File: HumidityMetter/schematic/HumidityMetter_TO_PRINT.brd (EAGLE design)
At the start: 100 x 68 mm, 66 parts, among them IC1 LM317, IC2 LM317, IC3 STM32F103C8T6, IC4 AM2320, J1 0, J2 0, J3 0, J4 0, K1 POWER_ON, T1 BSS84, T2 BC847, X1 +9V, X2 GND, X3 ISP

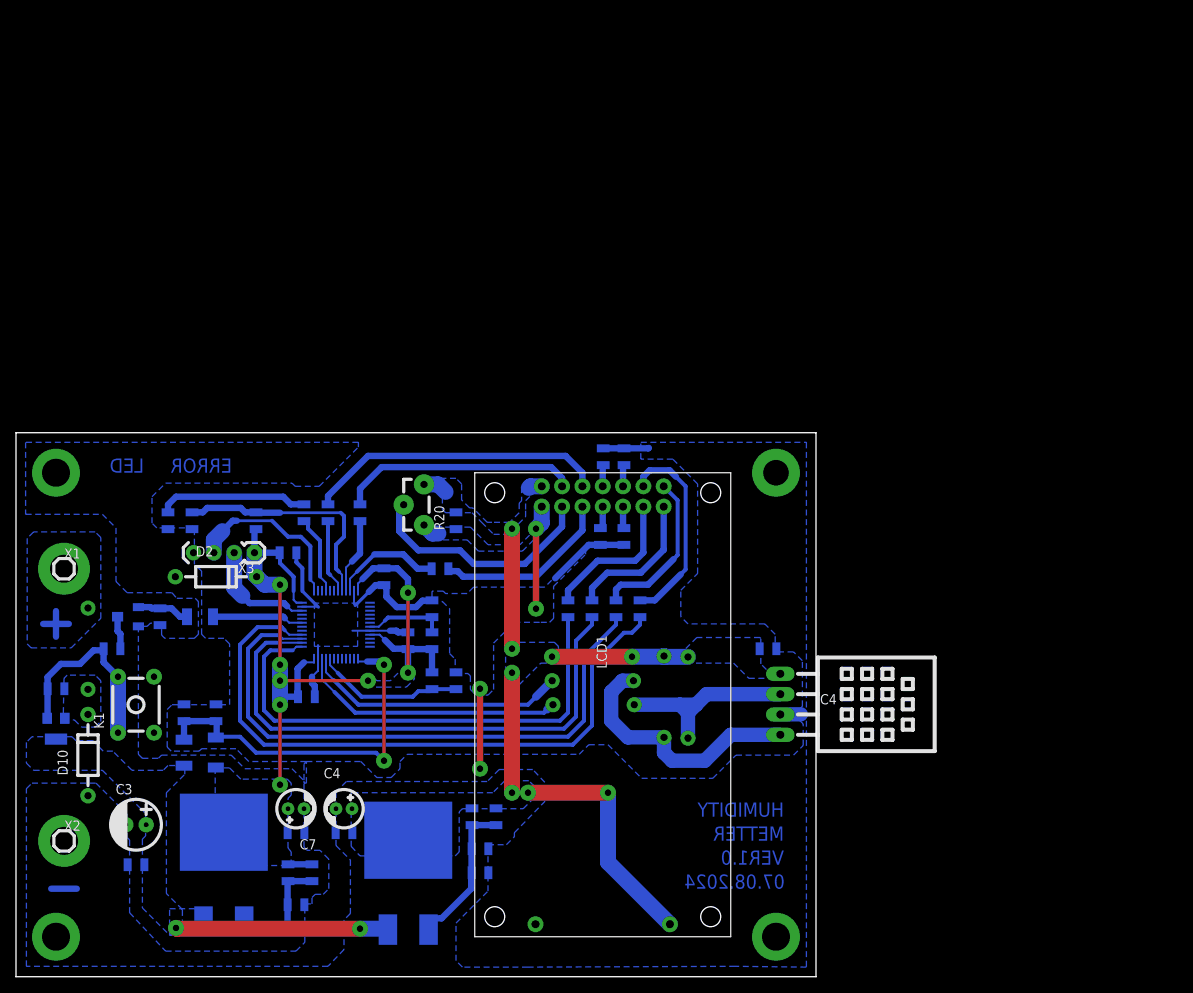
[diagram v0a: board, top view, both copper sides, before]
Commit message: Himidity metter. Board routed. Fix tiny problems.
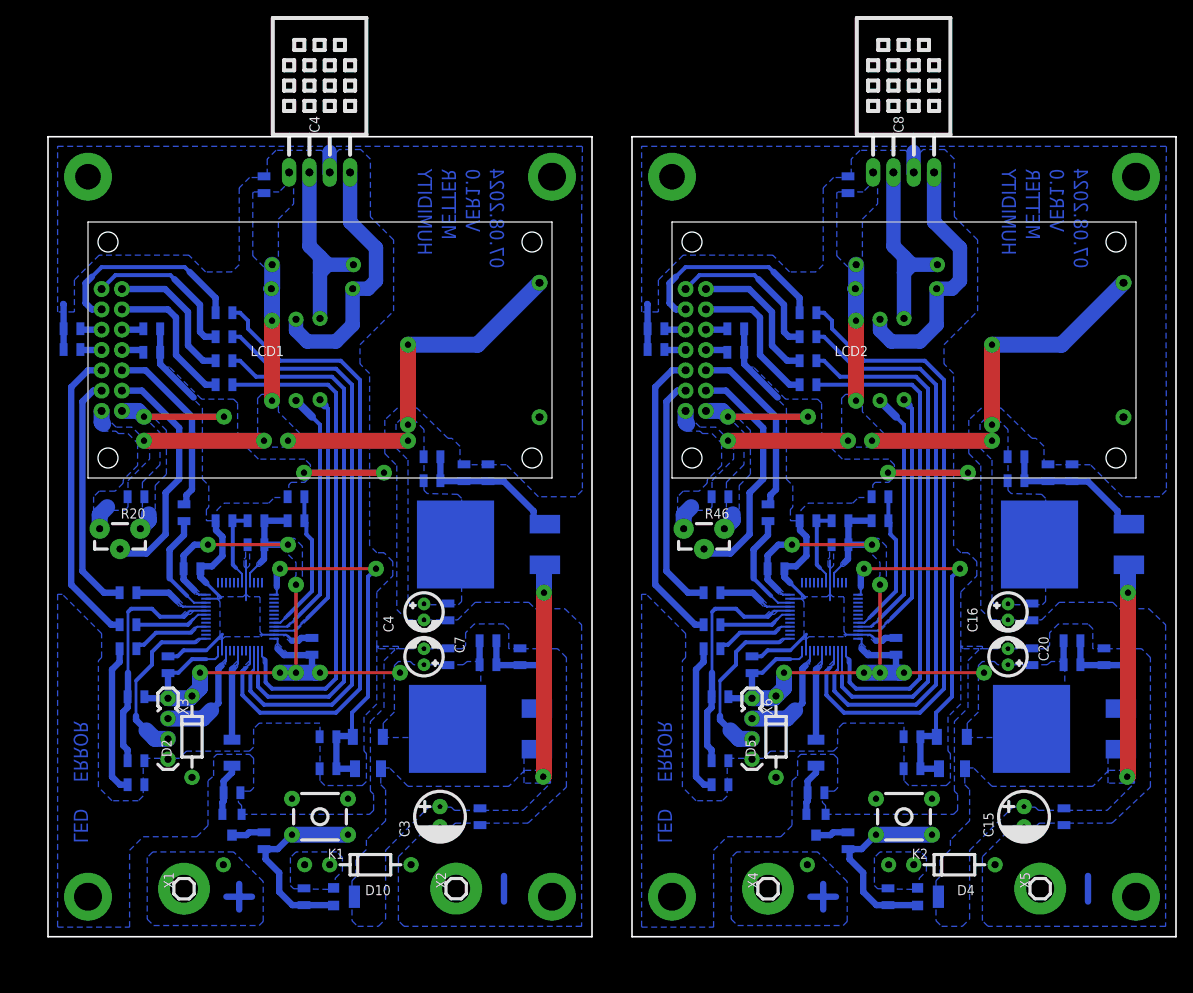
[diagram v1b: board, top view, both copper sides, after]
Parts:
- added C15: 100uFx16V, __MyCommonLib1:CE_6.3MM
- added C16, C20: 10uF x 10V, __MyCommonLib1:CE_5.2MM
- added C17, C18, C19, C21, C22, C23, C24, C25, C26, C27, C28: 0.1uF, __MyCommonLib1:RSMD_0805
- added D3: LL4148, __MyCommonLib1:SOD-80
- added D4, D5: 1N4007, __MyCommonLib1:DO-41_10MM
- added IC5: STM32F103C8T6, __MyCommonLib1:LQFP48
- added IC6, IC7: LM317, __MyCommonLib1:D2PAK
- added IC8: AM2320, __MyCommonLib1:AM2320_HOR
- added J5, J6, J7, J8: 0, __MyCommonLib1:RSMD_0805
- added K2: POWER_ON, __MyCommonLib1:KEY_7X4.5
- added LCD2: LCD_0802B, __MyCommonLib1:LCD_0802B(CHINA_CLONE)
- added LED2: ERROR(RED), __MyCommonLib1:LED_0805
- added R34: 1 Ohm, __MyCommonLib1:R0207
- added R35, R37, R59: 10K, __MyCommonLib1:RSMD_0805
- added R36, R38, R66: 1K0, __MyCommonLib1:RSMD_0805
- added R39: 3K0, __MyCommonLib1:RSMD_0805
- added R40, R43, R64, R65: *, __MyCommonLib1:RSMD_0805
- added R41: 3K9, __MyCommonLib1:RSMD_0805
- added R42: 2K2, __MyCommonLib1:RSMD_0805
- added R44: 1K0, __MyCommonLib1:RSMD_1206_BIG_GAP
- added R45, R47, R48, R49, R54, R55, R56: 390R, __MyCommonLib1:RSMD_0805
- added R46: 10K, __MyCommonLib1:R_ADJ_STAND
- added R50, R51, R52, R53: 2K0, __MyCommonLib1:RSMD_0805
- added R57: 18K, __MyCommonLib1:RSMD_1206_BIG_GAP
- added R58: 6K8, __MyCommonLib1:RSMD_0805
- added R60, R61: 4K7, __MyCommonLib1:R0207
- added R62, R63: 200R, __MyCommonLib1:R0207
- added T3: BSS84, __MyCommonLib1:SOT23
- added T4: BC847, __MyCommonLib1:SOT23_SMALL_PADS
- added X4: +9V, __MyCommonLib1:PIN1X1_D3.5MM
- added X5: GND, __MyCommonLib1:PIN1X1_D3.5MM
- added X6: ISP, __MyCommonLib1:PIN4X1_2.54MM
- moved IC4 94.3 mm to (34.0, 100.0), turned to 90 degrees
- moved C1 85.6 mm to (27.0, 94.0), turned to 270 degrees
- moved R26 71.6 mm to (33.1, 84.0), turned to 180 degrees
- moved R16 70.8 mm to (3.00, 76.0), turned to 0 degrees
- moved R18 67.7 mm to (3.00, 73.4), turned to 0 degrees
- moved R27 67.4 mm to (33.0, 81.0), turned to 180 degrees
- moved R17 64.5 mm to (13.0, 76.0), turned to 180 degrees
- moved R14 63.8 mm to (22.0, 78.0), turned to 180 degrees
- moved R19 60.6 mm to (13.0, 73.0), turned to 180 degrees
- moved R12 59.6 mm to (22.0, 75.0), turned to 180 degrees
- moved R13 55.5 mm to (22.0, 72.0), turned to 180 degrees
- moved R28 55.1 mm to (34.0, 72.2), turned to 90 degrees
- moved R29 54.6 mm to (31.0, 72.1), turned to 90 degrees
- moved R15 51.3 mm to (22.0, 69.0), turned to 180 degrees
- moved R6 50.0 mm to (55.0, 58.0), turned to 90 degrees
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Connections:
- new net +3.3V1: C19.PAD_1, C20.PLUS, C23.PAD_1, C24.PAD_1, C25.PAD_1, C26.PAD_1, D3.CATHODE, D5.CATHODE, IC5.24, IC5.36, IC5.48, IC5.9, IC7.2, J5.PAD_0, J7.PAD_0, R42.PAD_1, R59.PAD_0, R64.PAD_1, X6.1
- new net +5V1: C16.PLUS, C18.PAD_1, C21.PAD_1, C28.PAD_1, IC6.2, IC8.1, LCD2.2, LCD2.A, R38.PAD_1, R46.3, R60.PAD_0, R61.PAD_0, R65.PAD_1
- new net ADC_9V1: C22.PAD_1, D3.ANODE, IC5.13, R57.PAD_1, R58.PAD_0
- new net BOOT2: IC5.20, J7.PAD_1, J8.PAD_0
- new net BOOT3: IC5.44, J5.PAD_1, J6.PAD_0
- new net ERROR_LED1: IC5.40, R66.PAD_0
- new net GND1: C15.MINUS, C16.MINUS, C17.PAD_0, C18.PAD_0, C19.PAD_0, C20.MINUS, C21.PAD_0, C22.PAD_0, C23.PAD_0, C24.PAD_0, C25.PAD_0, C26.PAD_0, C27.PAD_0, C28.PAD_0, D4.ANODE, D5.ANODE, IC5.23, IC5.35, IC5.47, IC5.8, IC8.3, J6.PAD_1, J8.PAD_1, K2.1, K2.2, LCD2.1, LCD2.K, LED2.CATHODE, R37.PAD_1, R39.PAD_1, R40.PAD_1, R41.PAD_1, R43.PAD_1, R46.1, R50.PAD_1, R51.PAD_1, R52.PAD_1, R53.PAD_1, R58.PAD_1, T4.2, X5.1, X6.4
- new net I2C_SCL1: IC5.21, R63.PAD_0
- new net I2C_SDA1: IC5.22, R62.PAD_0
- new net LCD_D1: IC5.27, R45.PAD_1
- new net LCD_D2: IC5.26, R47.PAD_1
- new net LCD_D3: IC5.28, R48.PAD_1
- new net LCD_D8: IC5.25, R49.PAD_1
- new net LCD_E1: IC5.43, R54.PAD_1
- new net LCD_R/~W1: IC5.46, R55.PAD_1
- new net LCD_RS1: IC5.45, R56.PAD_1
- new net N$24: R34.PAD1, X4.1
- new net N$25: D4.CATHODE, R34.PAD_0, R35.PAD_0, T3.2
- new net N$26: K2.3, K2.4, R35.PAD_1, R36.PAD_0, T3.1
- new net N$27: R36.PAD_1, T4.3
- new net N$29: R37.PAD_0, R44.PAD_1, T4.1
- new net N$31: C15.PLUS, C17.PAD_1, IC6.3, IC7.3, R57.PAD_0, T3.3
- new net N$32: IC6.1, R38.PAD_0, R39.PAD_0, R40.PAD_0, R65.PAD_0
- new net N$33: IC7.1, R41.PAD_0, R42.PAD_0, R43.PAD_0, R64.PAD_0
- new net N$34: LCD2.14, R45.PAD_0
- new net N$35: LCD2.13, R47.PAD_0
- new net N$36: LCD2.12, R48.PAD_0
- new net N$37: LCD2.11, R49.PAD_0
- new net N$38: LCD2.10, R50.PAD_0
- new net N$39: LCD2.9, R51.PAD_0
- new net N$40: LCD2.8, R52.PAD_0
- new net N$41: LCD2.7, R53.PAD_0
- new net N$42: LCD2.4, R56.PAD_0
- new net N$43: LCD2.5, R55.PAD_0
- new net N$44: LCD2.6, R54.PAD_0
- new net N$45: IC8.2, R60.PAD1, R62.PAD1
- new net N$46: IC8.4, R61.PAD1, R63.PAD1
- new net N$47: LCD2.3, R46.2
- new net N$48: LED2.ANODE, R66.PAD_1
- new net NRST1: C27.PAD_1, IC5.7, R59.PAD_1
- new net PWR_HOLD1: IC5.31, R44.PAD_0
- new net SWDCLK1: IC5.37, X6.3
- new net SWDIO1: IC5.34, X6.2
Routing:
- net +3.3V1: track 0.00 -> 103.0 mm, vias 0 -> 8
- net +5V1: track 0.00 -> 81.5 mm, vias 0 -> 8
- net LCD_D3: track 0.00 -> 81.4 mm
- net GND1: track 0.00 -> 80.4 mm, vias 0 -> 8
- net LCD_D1: track 0.00 -> 74.6 mm
- net LCD_D2: track 0.00 -> 68.6 mm
- net LCD_D8: track 0.00 -> 62.9 mm
- net ADC_9V1: track 0.00 -> 46.4 mm, vias 0 -> 2
- net N$44: track 0.00 -> 37.5 mm
- net I2C_SDA1: track 0.00 -> 33.6 mm
- net I2C_SCL1: track 0.00 -> 32.9 mm
- net N$46: track 0.00 -> 32.6 mm
- net N$47: track 0.00 -> 30.0 mm
- net N$42: track 0.00 -> 29.9 mm
- net BOOT3: track 0.00 -> 29.7 mm
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- added copper zone on layer 16, net +3.3V1
- added copper zone on layer 16, net +5V1
- added copper zone on layer 16, net ADC_9V
- added copper zone on layer 16, net ADC_9V1
- added copper zone on layer 16, net BOOT0
- added copper zone on layer 16, net BOOT1
- added copper zone on layer 16, net BOOT2
- added copper zone on layer 16, net BOOT3
- added copper zone on layer 16, net ERROR_LED
- added copper zone on layer 16, net ERROR_LED1
- added copper zone on layer 16, net GND1
- added copper zone on layer 16, net I2C_SCL
- added copper zone on layer 16, net I2C_SCL1
- added copper zone on layer 16, net I2C_SDA
- added copper zone on layer 16, net I2C_SDA1
- added copper zone on layer 16, net LCD_D1
- added copper zone on layer 16, net LCD_D3
- added copper zone on layer 16, net LCD_D4
- added copper zone on layer 16, net LCD_D5
- added copper zone on layer 16, net LCD_D7
- added copper zone on layer 16, net LCD_D8
- added copper zone on layer 16, net LCD_E
- added copper zone on layer 16, net LCD_E1
- added copper zone on layer 16, net LCD_RS
- added copper zone on layer 16, net LCD_RS1
- added copper zone on layer 16, net N$24
- added copper zone on layer 16, net N$25
- added copper zone on layer 16, net N$31
- added copper zone on layer 16, net PWR_HOLD
- added copper zone on layer 16, net PWR_HOLD1
- added copper zone on layer 16, net SWDCLK
- added copper zone on layer 16, net SWDCLK1
- added copper zone on layer 16, net SWDIO
- added copper zone on layer 16, net SWDIO1
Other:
- board size 100 x 68 mm -> 141 x 100 mm
